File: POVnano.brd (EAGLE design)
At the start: 62.4 x 55.4 mm, 12 parts

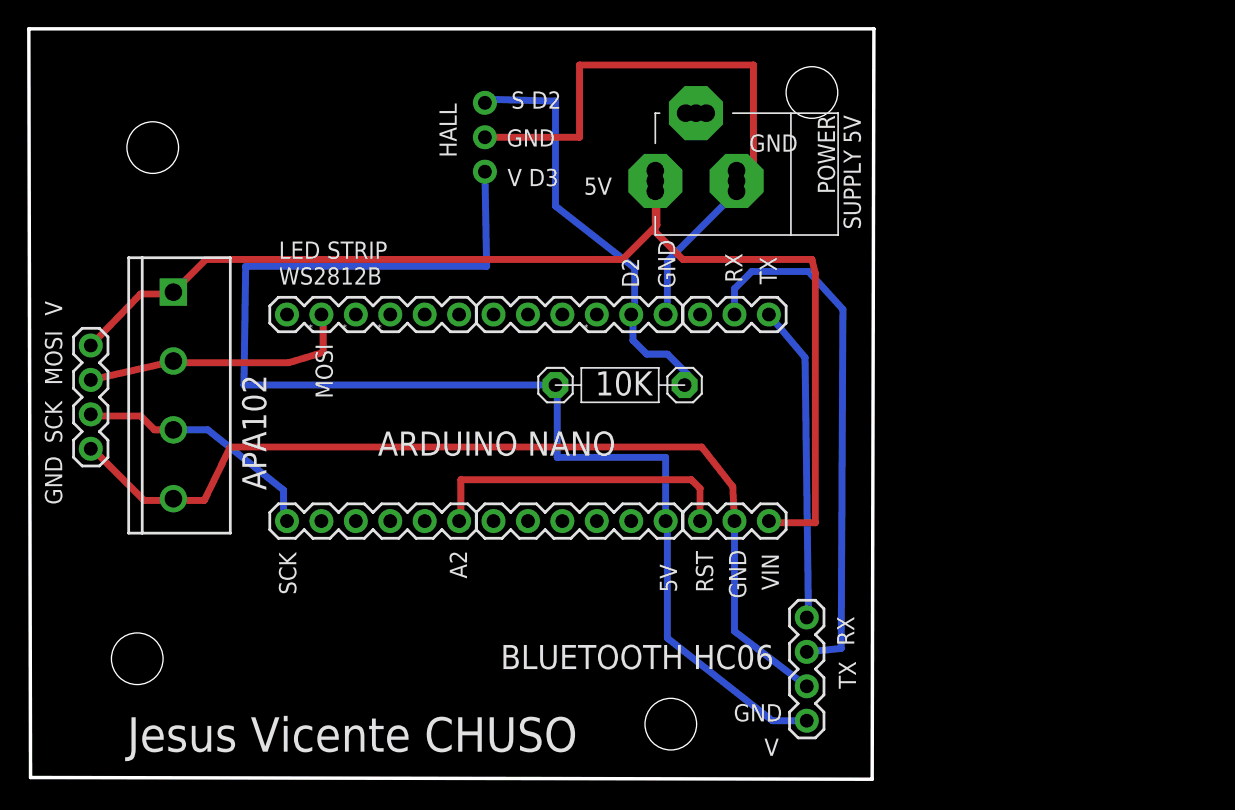
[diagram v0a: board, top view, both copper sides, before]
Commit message: sdfsd
sdf
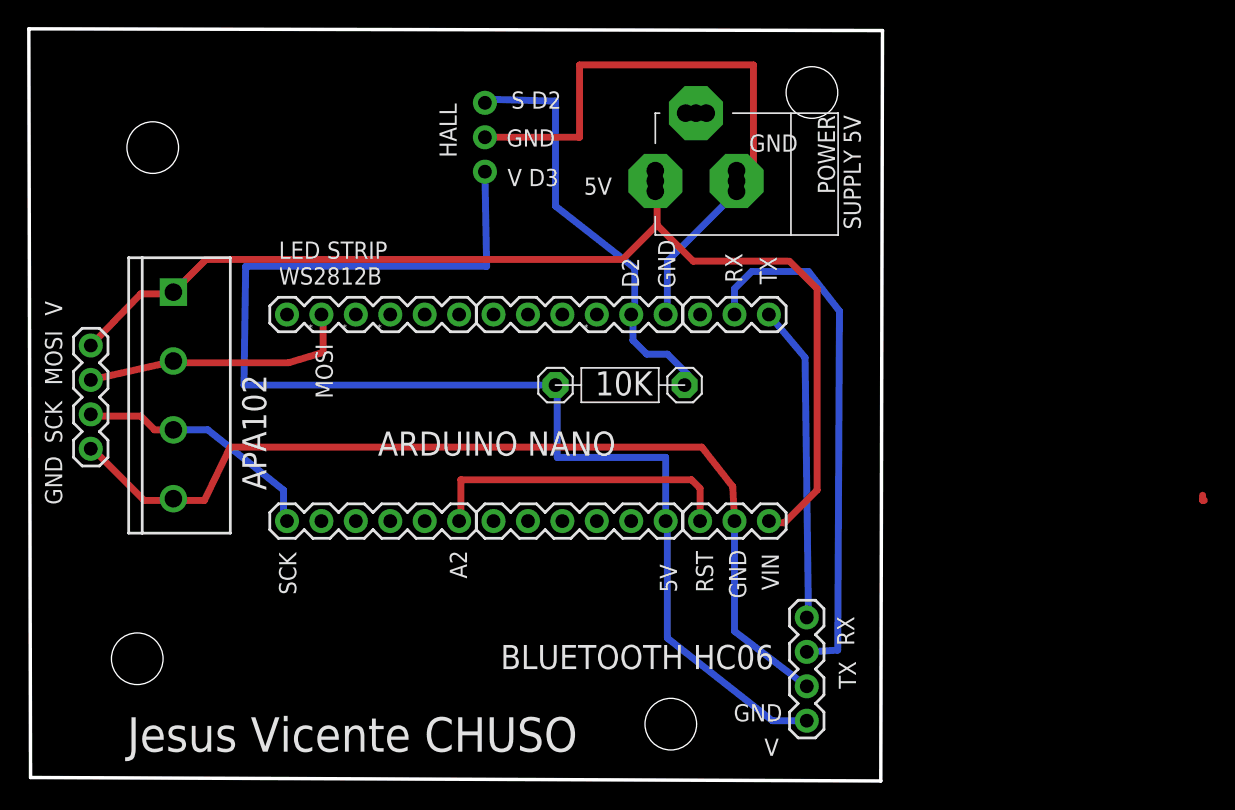
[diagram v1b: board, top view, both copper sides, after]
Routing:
- net S$8: track 0.00 -> 50.5 mm
- net S$6: track 39.7 -> 0.00 mm
- net S$9: track 35.8 -> 0.00 mm
- net S$21: track 0.00 -> 22.3 mm
- net S$7: track 3.43 -> 0.00 mm
- net S$32: track 0.00 -> 0.51 mm
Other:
- board size 62.4 x 55.4 mm -> 63 x 55.5 mm
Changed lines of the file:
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@@
 <text x="-16.1798" y="1.1938" size="0.508" layer="21" ratio="12">*</text>
 <text x="4.1402" y="1.1938" size="0.508" layer="21" ratio="12">*</text>
-<wire x1="-36.83" y1="23.495" x2="25.527" y2="23.495" width="0.254" layer="20"/>
-<wire x1="25.527" y1="23.495" x2="25.4" y2="-31.877" width="0.254" layer="20"/>
-<wire x1="25.4" y1="-31.877" x2="-36.703" y2="-31.75" width="0.254" layer="20"/>
+<wire x1="-36.83" y1="23.495" x2="26.162" y2="23.368" width="0.254" layer="20"/>
+<wire x1="26.162" y1="23.368" x2="26.035" y2="-32.004" width="0.254" layer="20"/>
+<wire x1="26.035" y1="-32.004" x2="-36.703" y2="-31.75" width="0.254" layer="20"/>
 <wire x1="-36.703" y1="-31.75" x2="-36.83" y2="23.495" width="0.254" layer="20"/>
 <text x="-19.304" y="-10.541" size="1.778" layer="25" font="vector" rot="R90">APA102</text>
@@
 <wire x1="-2.413" y1="2.286" x2="-2.54" y2="2.286" width="0.508" layer="1"/>
 </signal>
-<signal name="S$7">
-<wire x1="9.398" y1="12.573" x2="9.398" y2="9.144" width="0.508" layer="1"/>
-</signal>
-<signal name="S$9">
-<wire x1="9.398" y1="9.017" x2="9.398" y2="8.509" width="0.508" layer="1"/>
-<wire x1="9.398" y1="8.509" x2="11.43" y2="6.477" width="0.508" layer="1"/>
-<wire x1="11.43" y1="6.477" x2="20.955" y2="6.477" width="0.508" layer="1"/>
-<wire x1="20.955" y1="6.477" x2="21.209" y2="5.461" width="0.508" layer="1"/>
-<wire x1="21.209" y1="5.461" x2="21.209" y2="-12.954" width="0.508" layer="1"/>
-<wire x1="17.78" y1="-12.954" x2="21.209" y2="-12.954" width="0.508" layer="1"/>
-</signal>
 <signal name="S$10">
 <wire x1="15.748" y1="11.811" x2="10.287" y2="6.35" width="0.508" layer="16"/>
@@
 <wire x1="15.24" y1="4.318" x2="16.51" y2="5.588" width="0.508" layer="16"/>
 <wire x1="16.51" y1="5.588" x2="20.701" y2="5.588" width="0.508" layer="16"/>
-<wire x1="20.701" y1="5.588" x2="23.241" y2="2.794" width="0.508" layer="16"/>
-<wire x1="23.241" y1="2.794" x2="23.114" y2="-22.225" width="0.508" layer="16"/>
-<wire x1="23.114" y1="-22.225" x2="20.701" y2="-22.479" width="0.508" layer="16"/>
+<wire x1="20.701" y1="5.588" x2="22.987" y2="2.667" width="0.508" layer="16"/>
+<wire x1="22.987" y1="2.667" x2="22.86" y2="-22.352" width="0.508" layer="16"/>
+<wire x1="22.86" y1="-22.352" x2="20.701" y2="-22.479" width="0.508" layer="16"/>
 </signal>
 <signal name="S$19">
@@
 <wire x1="-3.175" y1="15.494" x2="-3.175" y2="15.367" width="0.508" layer="1"/>
 </signal>
-<signal name="S$6">
+<signal name="S$32">
+<wire x1="49.911" y1="-11.303" x2="49.784" y2="-11.303" width="0.508" layer="1"/>
+<wire x1="49.784" y1="-11.303" x2="49.784" y2="-10.922" width="0.508" layer="1"/>
+</signal>
+<signal name="S$21">
+<wire x1="21.336" y1="4.318" x2="19.304" y2="6.35" width="0.508" layer="1"/>
+<wire x1="21.336" y1="-10.541" x2="21.336" y2="4.318" width="0.508" layer="1"/>
+<wire x1="17.78" y1="-12.954" x2="18.923" y2="-12.954" width="0.508" layer="1"/>
+<wire x1="18.923" y1="-12.954" x2="21.336" y2="-10.541" width="0.508" layer="1"/>
+</signal>
+<signal name="S$8">
 <wire x1="9.525" y1="11.176" x2="9.525" y2="9.017" width="0.508" layer="1"/>
 <wire x1="9.525" y1="9.017" x2="6.985" y2="6.477" width="0.508" layer="1"/>
 <wire x1="6.985" y1="6.477" x2="-23.749" y2="6.477" width="0.508" layer="1"/>
 <wire x1="-23.749" y1="6.477" x2="-26.035" y2="4.191" width="0.508" layer="1"/>
+<wire x1="19.177" y1="6.35" x2="12.192" y2="6.35" width="0.508" layer="1"/>
+<wire x1="12.192" y1="6.35" x2="9.525" y2="9.017" width="0.508" layer="1"/>
 </signal>
 </signals>
